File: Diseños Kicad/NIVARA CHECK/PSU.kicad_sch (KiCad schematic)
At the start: 10 parts, among them U2 AP63200WU

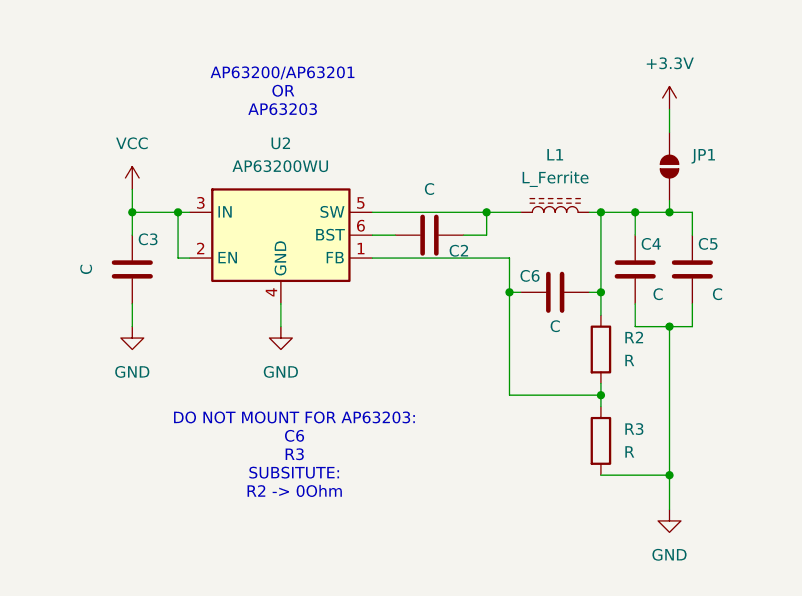
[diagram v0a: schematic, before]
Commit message: ACTUALIZACION HECHA
PCB SUPUESTA
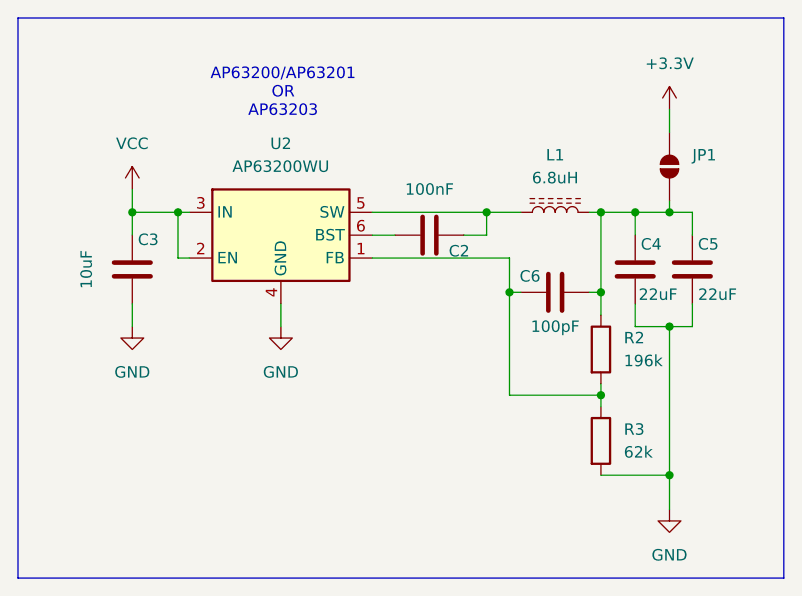
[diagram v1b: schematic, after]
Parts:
- C2: value C -> 100nF
- C3: value C -> 10uF
- C4, C5: value C -> 22uF
- C6: value C -> 100pF
- L1: value L_Ferrite -> 6.8uH
- R2: value R -> 196k
- R3: value R -> 62k
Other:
- note removed: "DO NOT MOUNT FOR AP63203: C6 R3 SUBSITUTE: R2 -> 0Ohm"
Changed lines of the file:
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@@
 	(generator_version "9.0")
 	(paper "A4")
-	(text "DO NOT MOUNT FOR AP63203:\nC6\nR3\nSUBSITUTE:\nR2 -> 0Ohm"
-		(exclude_from_sim no)
-		(at 49.784 67.818 0)
-		(effects
-			(font
-				(size 1.27 1.27)
-			)
+	(rectangle
+		(start 19.05 19.05)
+		(end 104.14 81.28)
+		(stroke
+			(width 0)
+			(type default)
+		)
+		(fill
+			(type none)
 		)
 	)
@@
 			)
 		)
-		(property "Value" "C"
+		(property "Value" "100pF"
 			(at 78.74 53.34 90)
 			(effects
@@
 			)
 		)
-		(property "Value" "C"
+		(property "Value" "22uF"
 			(at 90.17 49.784 0)
 			(effects
@@
 			)
 		)
-		(property "Value" "R"
+		(property "Value" "62k"
 			(at 86.36 67.3099 0)
 			(effects
@@
 			)
 		)
-		(property "Value" "R"
+		(property "Value" "196k"
 			(at 86.36 57.1499 0)
 			(effects
@@
 			)
 		)
-		(property "Value" "C"
+		(property "Value" "100nF"
 			(at 64.77 38.1 90)
 			(effects
@@
 			)
 		)
-		(property "Value" "C"
+		(property "Value" "22uF"
 			(at 96.774 49.784 0)
 			(effects
@@
 			)
 		)
-		(property "Value" "C"
+		(property "Value" "10uF"
 			(at 26.67 46.99 90)
 			(effects
@@
 			)
 		)
-		(property "Value" "L_Ferrite"
+		(property "Value" "6.8uH"
 			(at 78.74 36.83 90)
 			(effects
